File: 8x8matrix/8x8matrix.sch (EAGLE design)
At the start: 7 parts

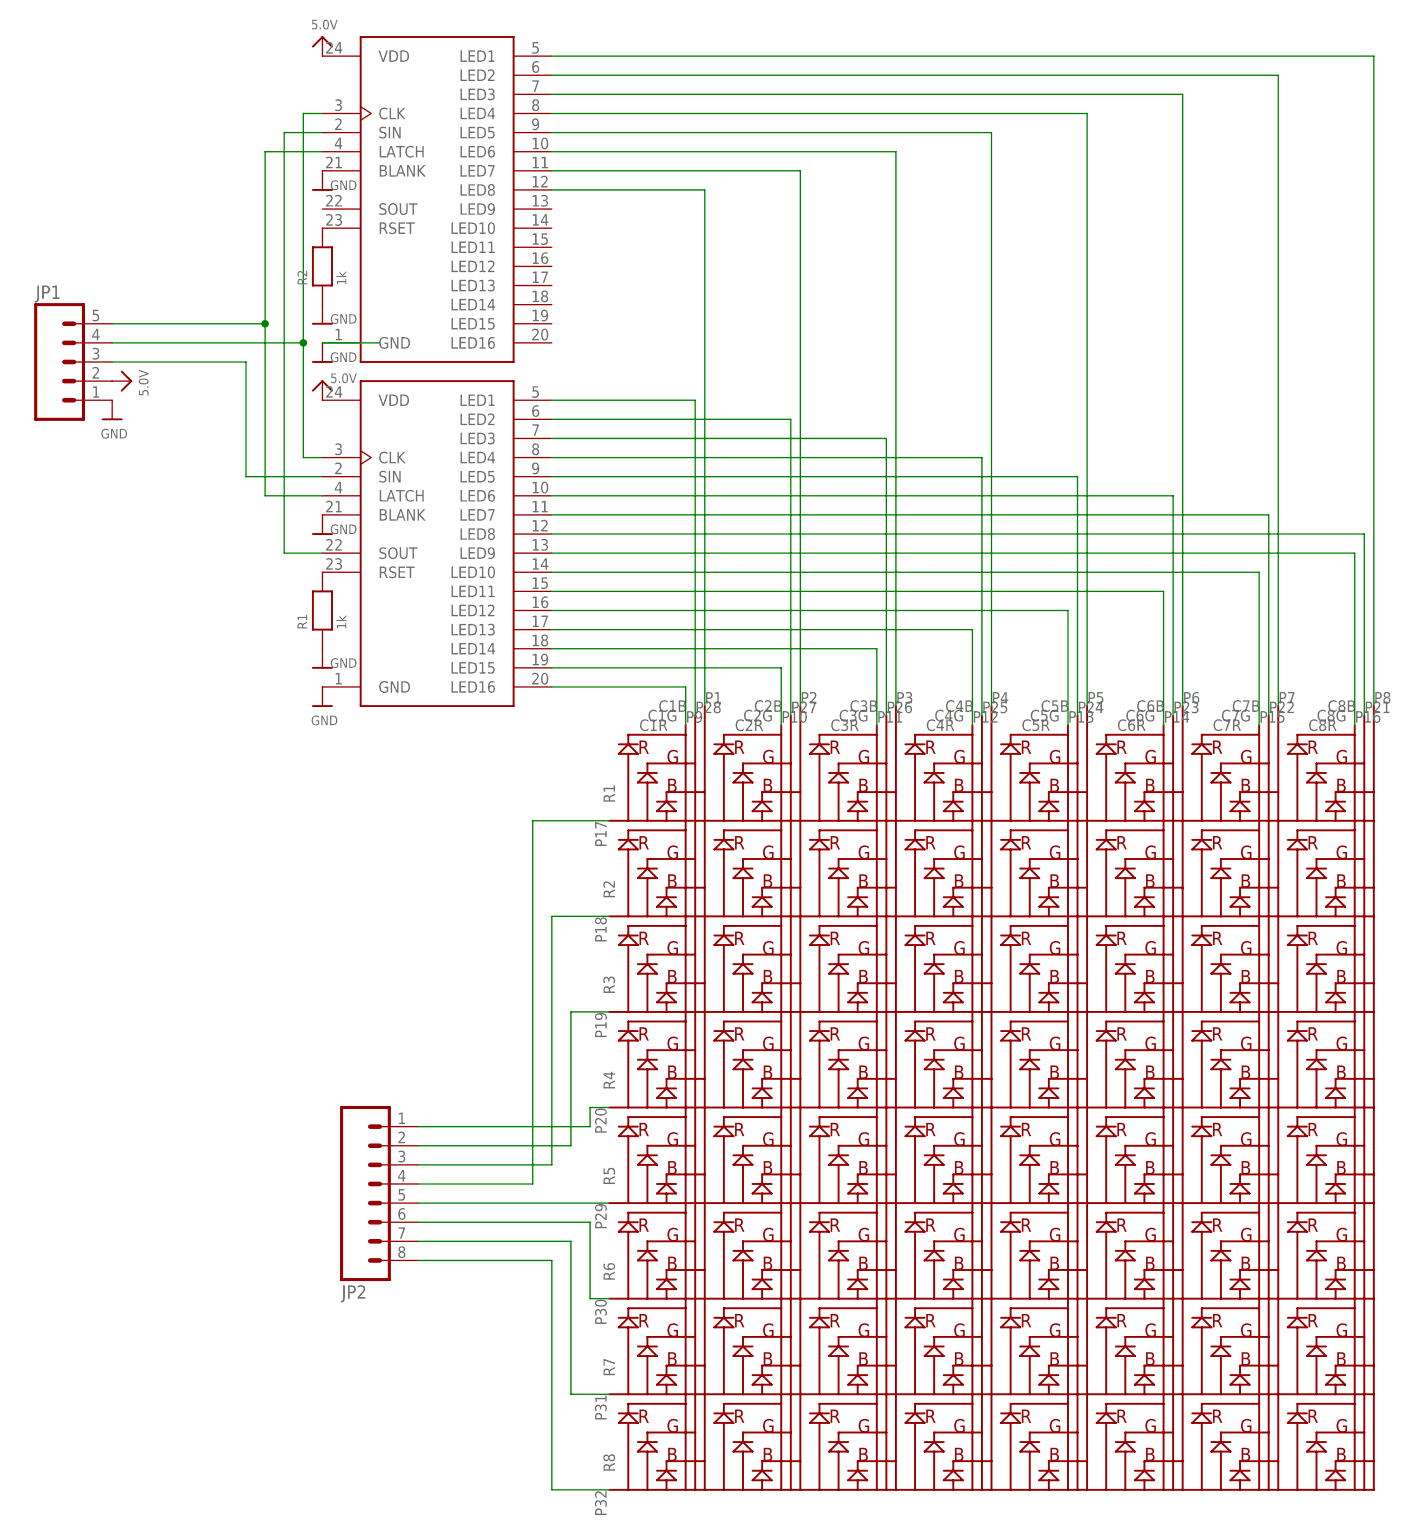
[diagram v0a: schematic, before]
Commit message: tlc
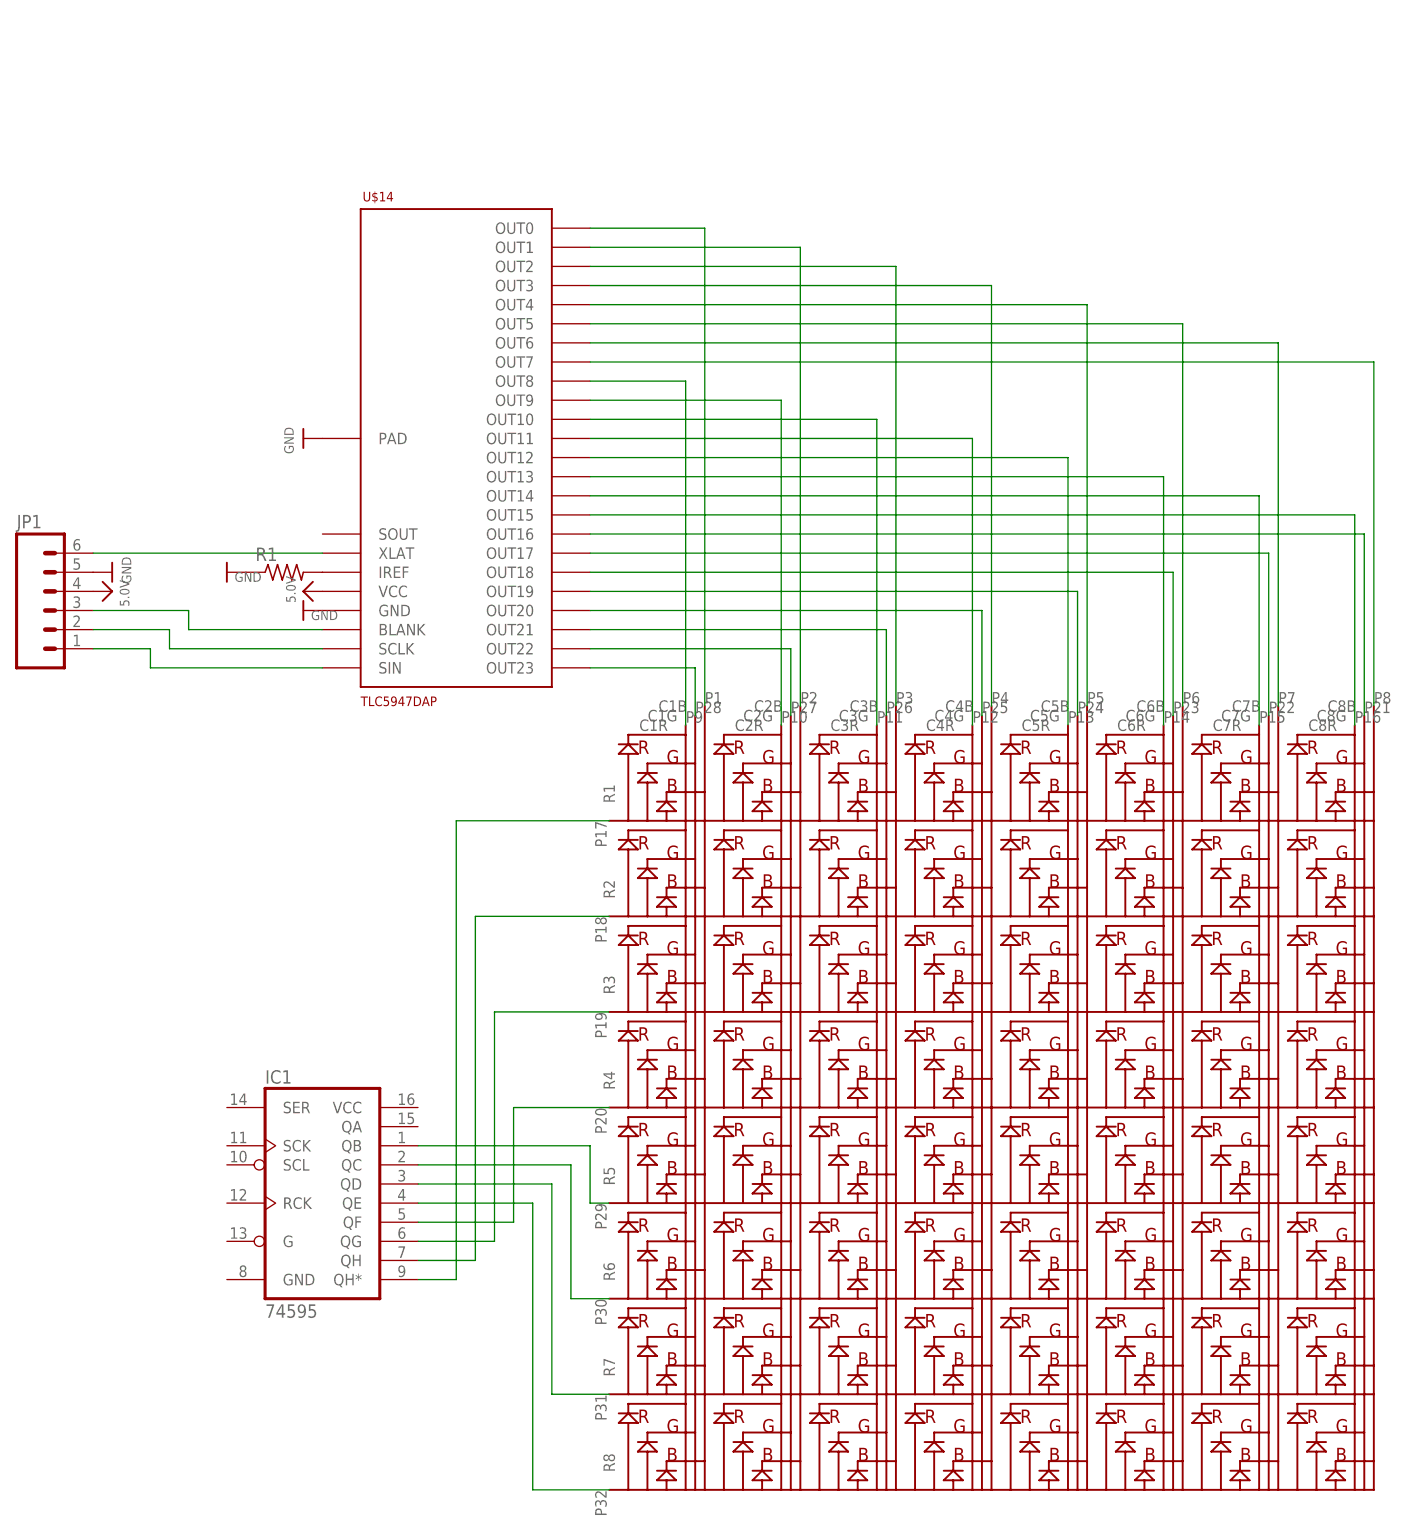
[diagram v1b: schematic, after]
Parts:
- removed JP2: (no value), SparkFun-Connectors:M081X08
- removed R2: 1k, microbuilder:RESISTOR0805_NOTHERMALS
- removed U$2, U$3: CAT4016W, CAT4016:CAT4016W
- added IC1: 74595, SparkFun-DigitalIC:74595
- added U$14: TLC5947DAP, TLC5947:TLC5947DAP
- JP1: device SparkFun-Connectors:M05PTH -> SparkFun-Connectors:M06SIP
- R1: value 1k -> (none); device microbuilder:RESISTOR0805_NOTHERMALS -> resistor:R-US_R0805
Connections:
- removed net CLK: JP1.4, U$2.CLK, U$3.CLK
- removed net LATCH: JP1.5, U$2.LATCH, U$3.LATCH
- removed net N$35: JP2.8, U$1.R8
- removed net SOUT: U$2.SIN, U$3.SOUT
- new net BLANK: JP1.3, U$14.BLANK
- new net N$27: R1.2, U$14.IREF
- new net XLAT: JP1.6, U$14.XLAT
- net 5.0V: now also JP1.4, U$14.VCC; no longer JP1.2, U$2.VDD, U$3.VDD
- net GND: now also JP1.5, U$14.GND, U$14.PAD; no longer JP1.1, R2.1, U$2.BLANK, U$2.GND, U$3.BLANK, U$3.GND
- net N$1: now also U$1.C1B, U$14.OUT0; no longer U$1.C8B, U$2.LED1
- net N$10: now also U$1.C2R, U$14.OUT9; no longer U$1.C2G, U$3.LED2
- net N$11: now also U$1.C3R, U$14.OUT10; no longer U$1.C3G, U$3.LED3
- net N$12: now also U$1.C4R, U$14.OUT11; no longer U$1.C4G, U$3.LED4
- net N$13: now also U$1.C5R, U$14.OUT12; no longer U$1.C5G, U$3.LED5
- net N$14: now also U$1.C6R, U$14.OUT13; no longer U$1.C6G, U$3.LED6
- net N$15: now also U$1.C7R, U$14.OUT14; no longer U$1.C7G, U$3.LED7
- net N$16: now also U$1.C8R, U$14.OUT15; no longer U$1.C8G, U$3.LED8
- net N$17: now also U$1.C8G, U$14.OUT16; no longer U$1.C8R, U$3.LED9
- net N$18: now also U$1.C7G, U$14.OUT17; no longer U$1.C7R, U$3.LED10
- net N$19: now also U$1.C6G, U$14.OUT18; no longer U$1.C6R, U$3.LED11
- net N$2: now also U$1.C2B, U$14.OUT1; no longer U$1.C7B, U$2.LED2
- net N$20: now also U$1.C5G, U$14.OUT19; no longer U$1.C5R, U$3.LED12
- net N$21: now also U$1.C4G, U$14.OUT20; no longer U$1.C4R, U$3.LED13
- net N$22: now also U$1.C3G, U$14.OUT21; no longer U$1.C3R, U$3.LED14
- net N$23: now also U$1.C2G, U$14.OUT22; no longer U$1.C2R, U$3.LED15
- net N$24: now also U$1.C1G, U$14.OUT23; no longer U$1.C1R, U$3.LED16
- net N$25: now also IC1.QB; no longer JP2.5
- net N$26: now also IC1.QC, U$1.R6; no longer JP2.1, U$1.R4
- net N$28: now also JP1.2, U$14.SCLK; no longer R1.2, U$3.RSET
- net N$29: now also IC1.QD, U$1.R7; no longer R2.2, U$2.RSET
- net N$3: now also U$1.C3B, U$14.OUT2; no longer U$1.C6B, U$2.LED3
- net N$30: now also IC1.QE, U$1.R8; no longer JP2.2, U$1.R3
- net N$31: now also IC1.QF, U$1.R4; no longer JP2.3, U$1.R2
- net N$32: now also IC1.QG, U$1.R3; no longer JP2.4, U$1.R1
- net N$33: now also IC1.QH, U$1.R2; no longer JP2.6, U$1.R6
- net N$34: now also IC1.QH*, U$1.R1; no longer JP2.7, U$1.R7
- net N$4: now also U$1.C4B, U$14.OUT3; no longer U$1.C5B, U$2.LED4
- net N$5: now also U$1.C5B, U$14.OUT4; no longer U$1.C4B, U$2.LED5
- net N$6: now also U$1.C6B, U$14.OUT5; no longer U$1.C3B, U$2.LED6
- net N$7: now also U$1.C7B, U$14.OUT6; no longer U$1.C2B, U$2.LED7
- net N$8: now also U$1.C8B, U$14.OUT7; no longer U$1.C1B, U$2.LED8
- net N$9: now also U$1.C1R, U$14.OUT8; no longer U$1.C1G, U$3.LED1
- net SIN: now also JP1.1, U$14.SIN; no longer JP1.3, U$3.SIN
